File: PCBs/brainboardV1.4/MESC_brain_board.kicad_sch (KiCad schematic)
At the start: 17 parts, among them J1 Conn_01x18, Q21 my_BC337, U21 Teensy4.0

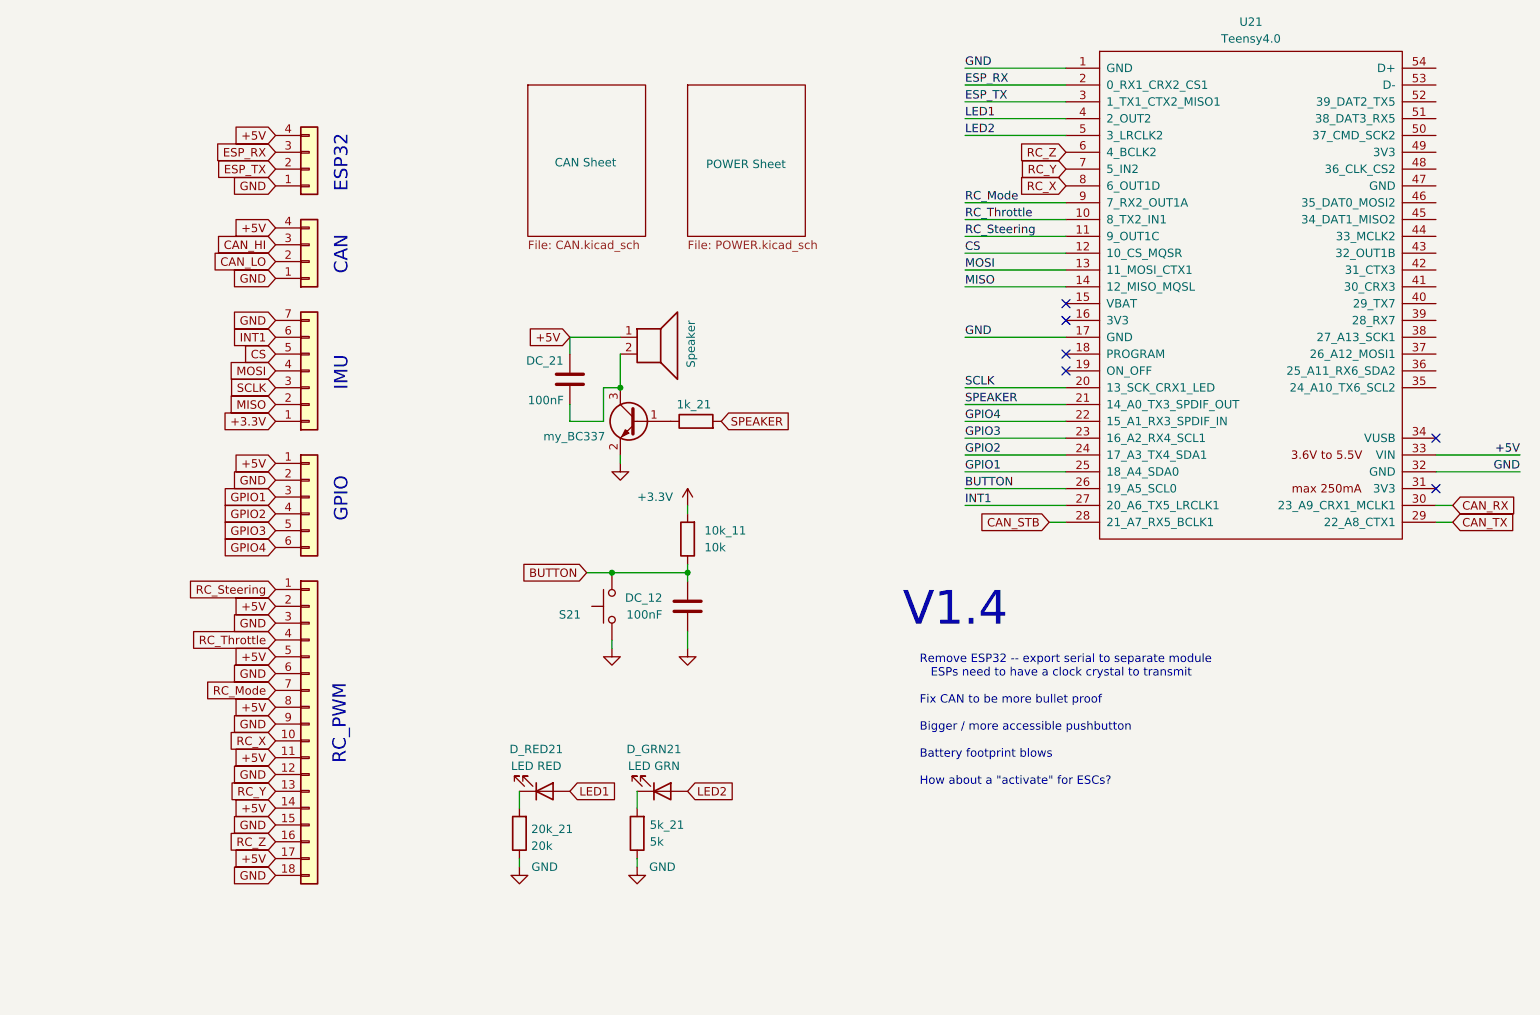
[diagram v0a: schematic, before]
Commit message: finalization of BB V1.4
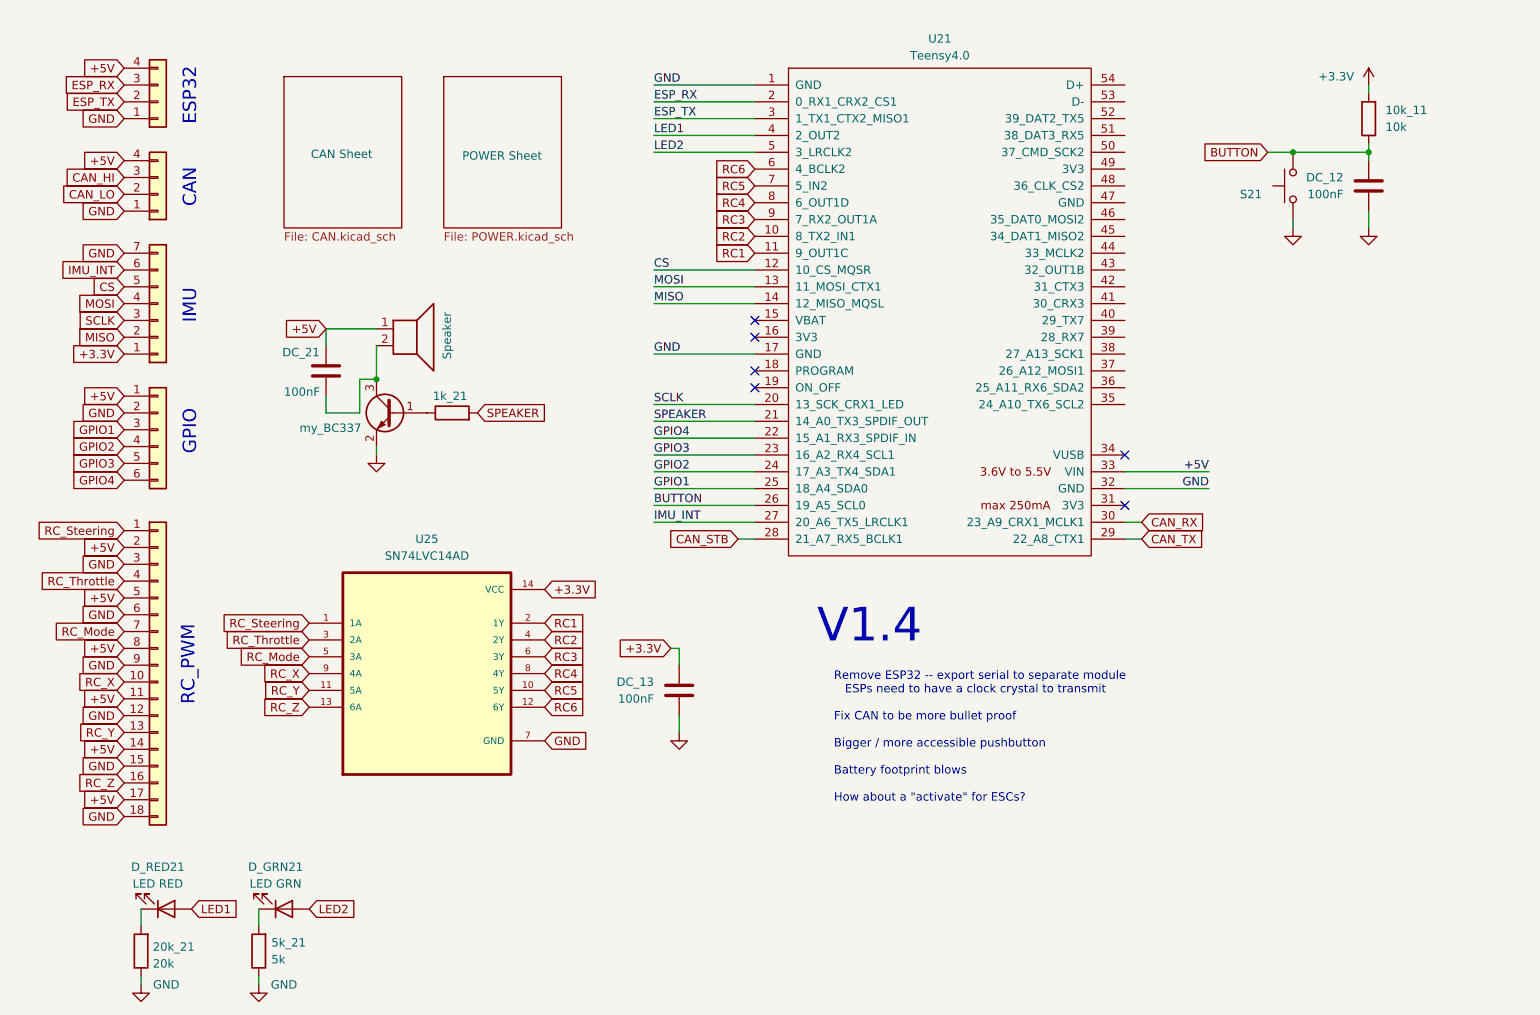
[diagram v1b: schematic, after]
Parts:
- added DC_13: 100nF, Capacitor_SMD:C_0603_1608Metric, symbol Device:C
- added U25: SN74LVC14AD, SN74LVC14AD:SOIC127P600X175-14N, symbol SN74LVC14AD:SN74LVC14AD
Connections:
- net +3.3V: now also DC_13.2, U25.14 (VCC)
- net GND: now also DC_13.1, U25.7 (GND)
- net RC_Mode: now also U25.5 (3A); no longer U21.9 (7_RX2_OUT1A)
- net RC_Steering: now also U25.1 (1A); no longer U21.11 (9_OUT1C)
- net RC_Throttle: now also U25.3 (2A); no longer U21.10 (8_TX2_IN1)
- net RC_X: now also U25.9 (4A); no longer U21.8 (6_OUT1D)
- net RC_Y: now also U25.11 (5A); no longer U21.7 (5_IN2)
- net RC_Z: now also U25.13 (6A); no longer U21.6 (4_BCLK2)
- net INT1 renamed IMU_INT
- new net RC1: U21.11 (9_OUT1C), U25.2 (1Y)
- new net RC2: U21.10 (8_TX2_IN1), U25.4 (2Y)
- new net RC3: U21.9 (7_RX2_OUT1A), U25.6 (3Y)
- new net RC4: U21.8 (6_OUT1D), U25.8 (4Y)
- new net RC5: U21.7 (5_IN2), U25.10 (5Y)
- new net RC6: U21.6 (4_BCLK2), U25.12 (6Y)
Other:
- moved on the sheet: 10k_11, 1k_21, 20k_21, 5k_21, DC_12, DC_21, D_GRN21, D_RED21, S21, U21

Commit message: encoder work
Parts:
- renumbered Q21 to Q1
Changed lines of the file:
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@@
 		(on_board yes)
 		(dnp no)
-		(property "Reference" "Q21"
+		(property "Reference" "Q1"
 			(at 63.5 69.8499 0)
 			(effects
@@
 			(project "MESC_brain_board"
 				(path "/8920b97c-b80b-47c5-aaa4-fe68c48cd11a"
-					(reference "Q21")
+					(reference "Q1")
 					(unit 1)
 				)
